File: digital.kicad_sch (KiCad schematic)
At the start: 30 parts

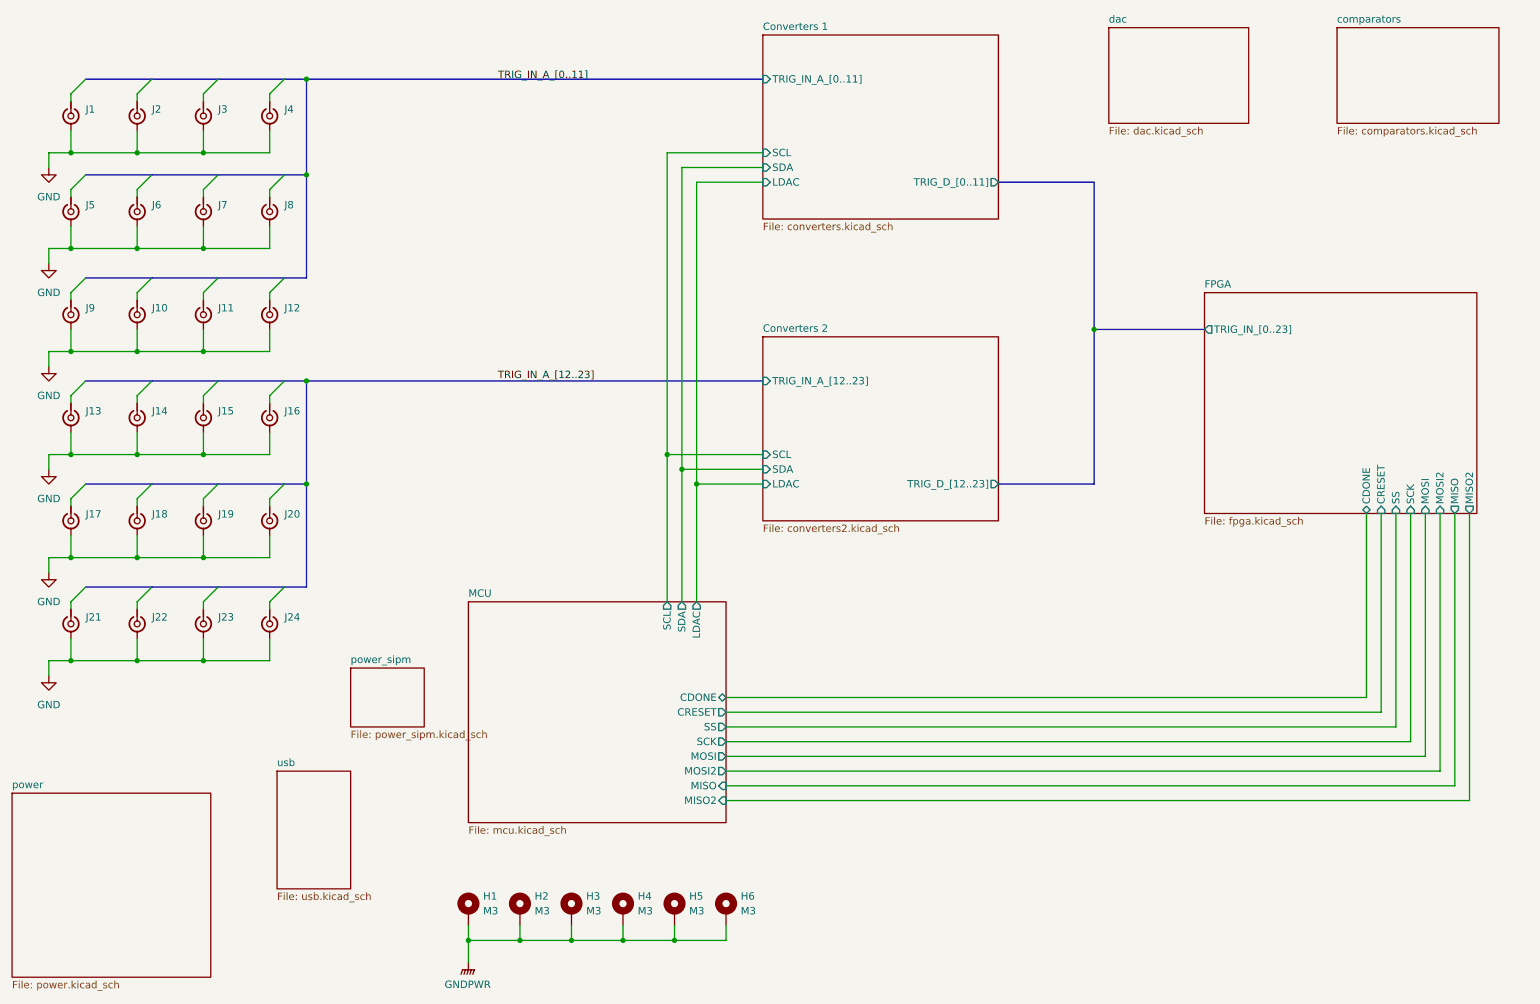
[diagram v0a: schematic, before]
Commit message: cleanup
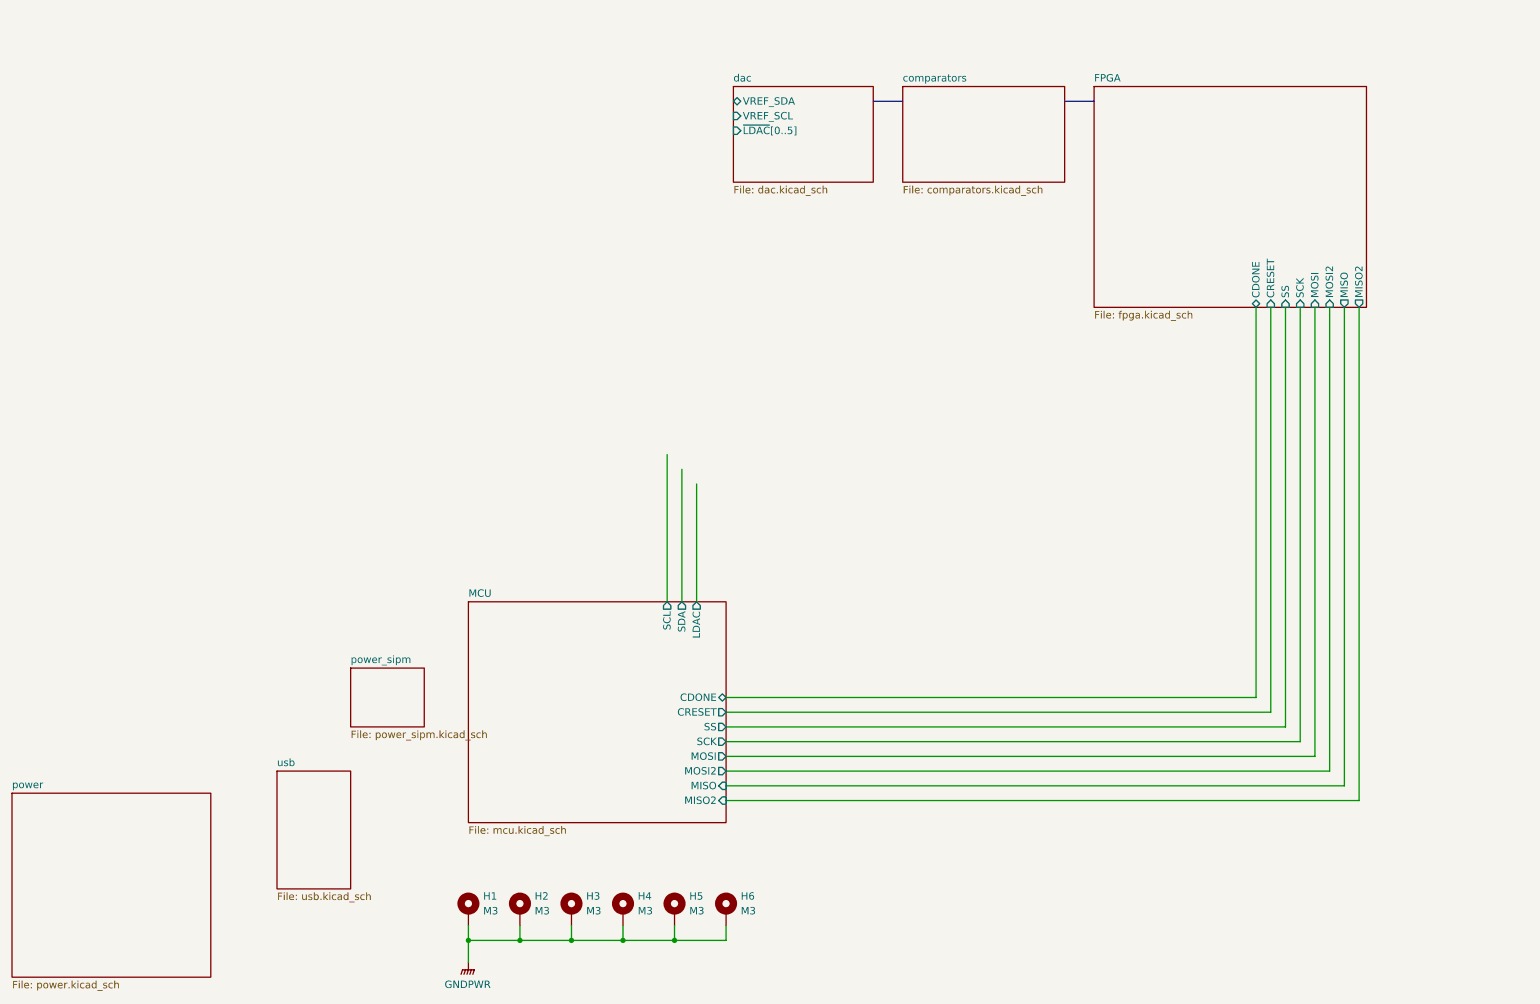
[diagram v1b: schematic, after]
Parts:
- removed J1, J10, J11, J12, J13, J14, J15, J16, J17, J18, J19, J2, J20, J21, J22, J23, J24, J3, J4, J5, J6, J7, J8, J9: ~, symbol Connector:Conn_Coaxial_Small
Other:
- removed sheet Converters 1
- removed sheet Converters 2
- sheet FPGA ports: added none; removed TRIG_IN_[0..23]
- sheet dac ports: added VREF_SCL, VREF_SDA, ~{LDAC}[0..5]; removed none

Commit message: rewire
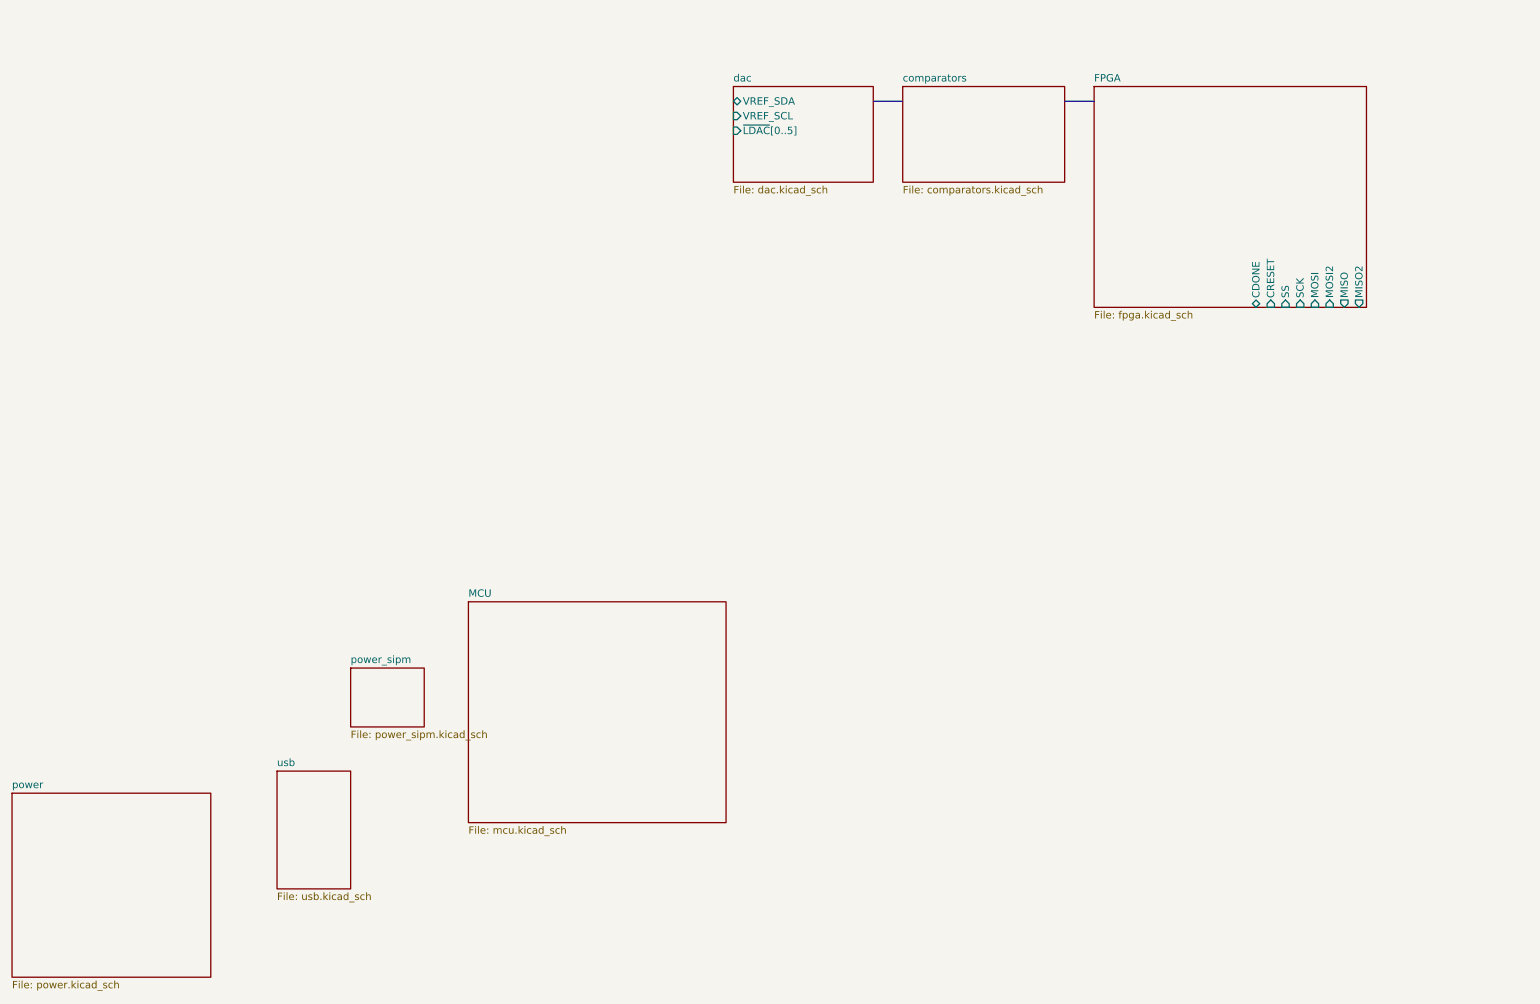
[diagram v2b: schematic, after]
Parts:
- removed H1, H2, H3, H4, H5, H6: M3, symbol Mechanical:MountingHole_Pad
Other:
- sheet MCU ports: added none; removed CDONE, CRESET, LDAC, MISO, MISO2, MOSI, MOSI2, SCK, SCL, SDA, SS
